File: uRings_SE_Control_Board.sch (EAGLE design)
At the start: 32 parts, among them J1 JACK-THONKICONN, J10 JACK-THONKICONN, J2 JACK-THONKICONN, J3 JACK-THONKICONN, J4 JACK-THONKICONN, J5 JACK-THONKICONN, J6 JACK-THONKICONN, J7 JACK-THONKICONN, J8 JACK-THONKICONN, J9 JACK-THONKICONN, P1 10k, P10 10k, P2 10k, P3 10k, P4 10k, P5 10k, P6 10k, P7 10k, P8 10k, P9 10k

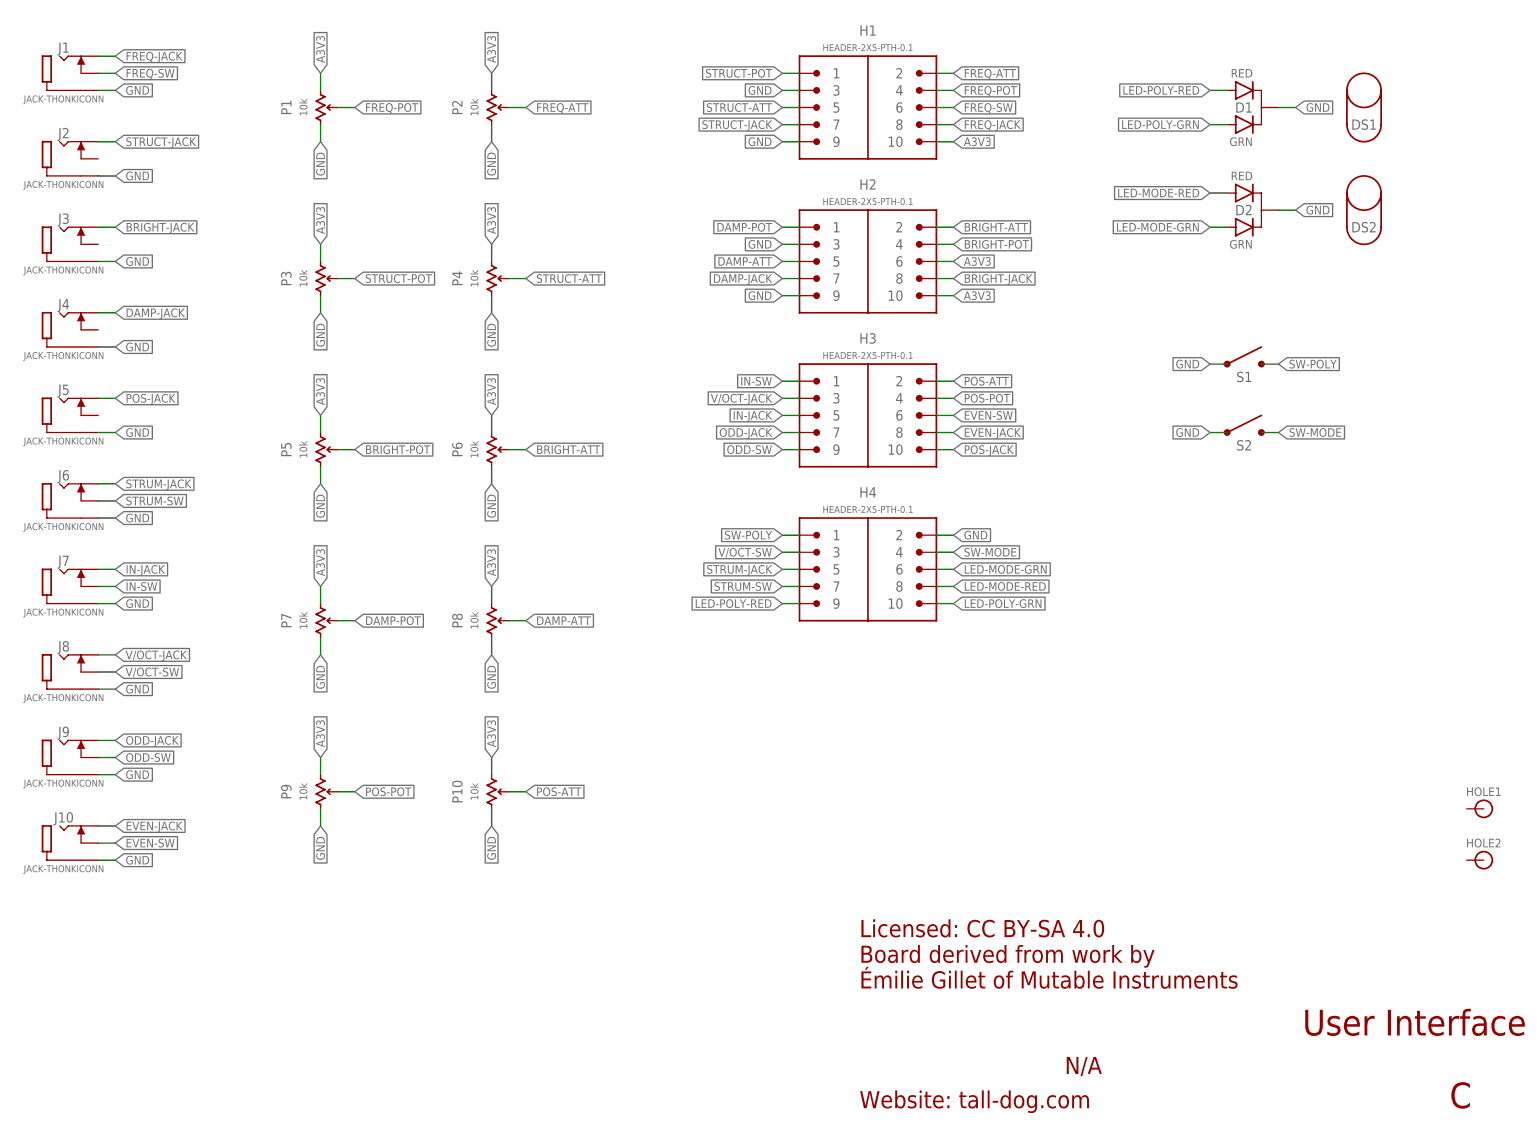
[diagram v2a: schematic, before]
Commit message: updates in preparation for rev D production
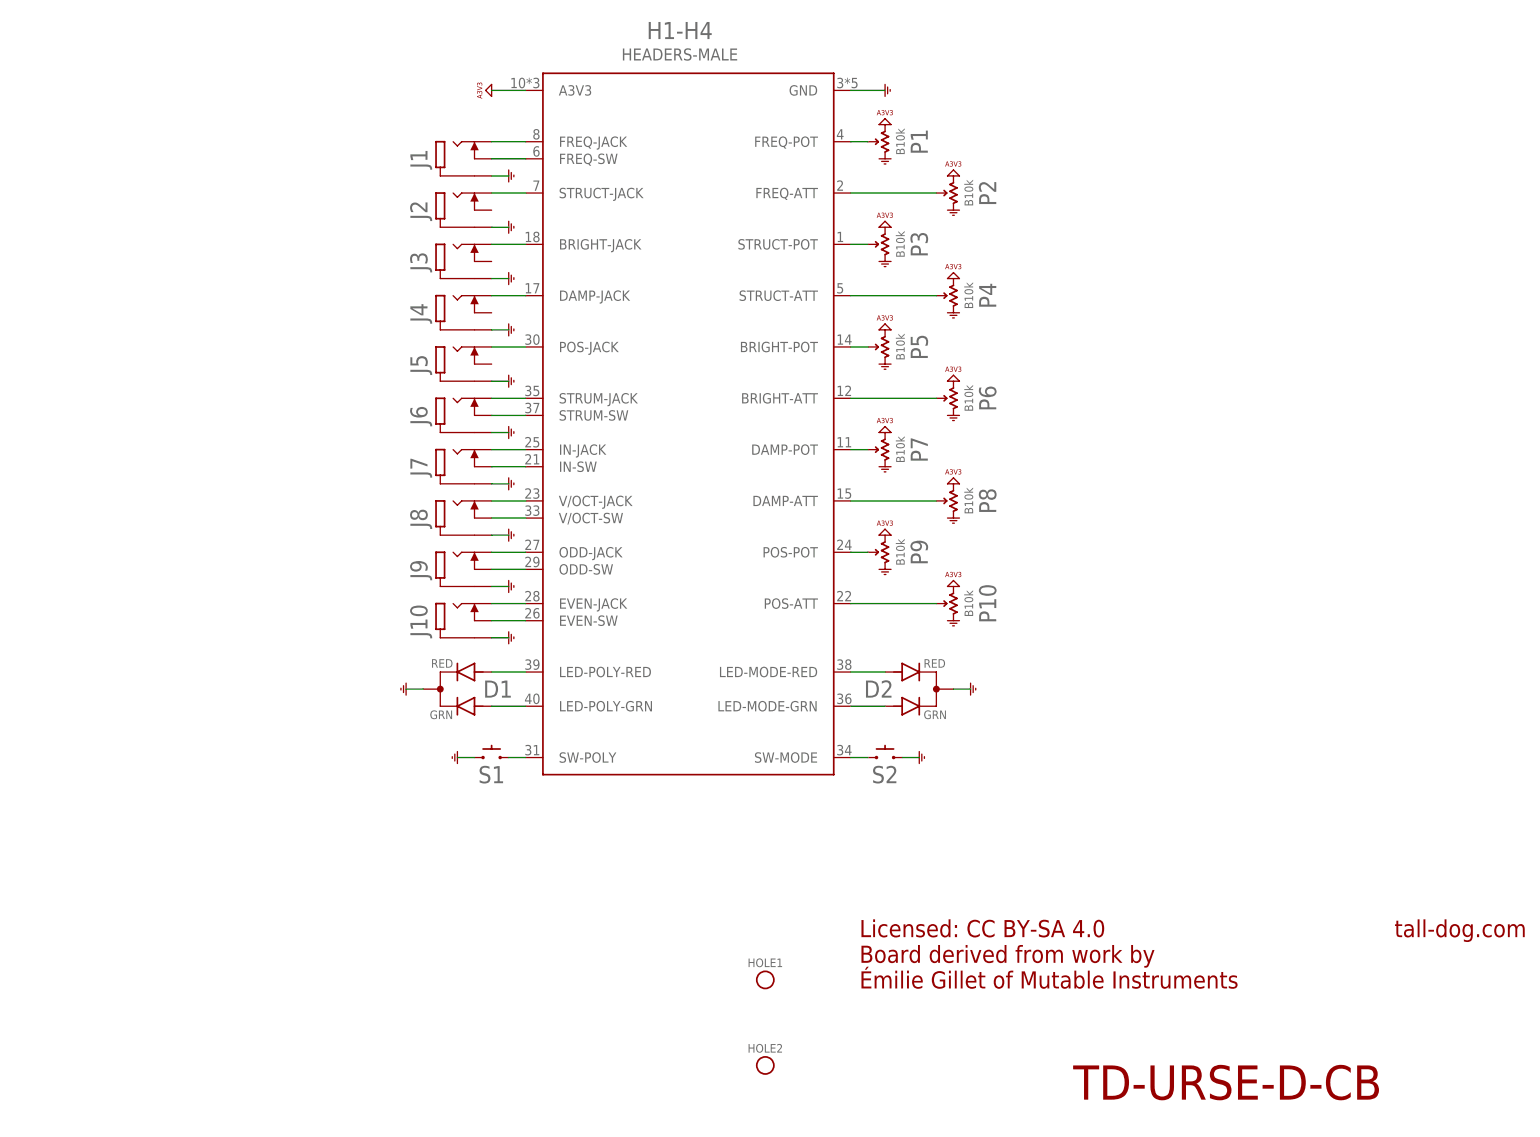
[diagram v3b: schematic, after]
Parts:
- removed DS1, DS2: LED-SPACER, uRings_SE_Library:LED-SPACER
- removed H1, H2, H3, H4: HEADER-2X5-PTH-0.1, uRings_SE_Library:HEADER-2X5-PTH-0.1
- added H1-H4: HEADERS-MALE, uRings_SE_Library:HEADERS-MALE
- D1, D2: value LED-DUAL-PTH -> LED-DUAL; device uRings_SE_Library:LED-DUAL-PTH -> uRings_SE_Library:LED-DUAL
- J1, J10, J2, J3, J4, J5, J6, J7, J8, J9: value JACK-THONKICONN -> JACK; device uRings_SE_Library:JACK-THONKICONN -> uRings_SE_Library:JACK
- P1, P10, P2, P3, P4, P5, P6, P7, P8, P9: value 10k -> B10k; device uRings_SE_Library:POT-ALPS-VERT-PS -> uRings_SE_Library:POT
- S1, S2: value SPST-PTH -> SPST; device uRings_SE_Library:SPST-PTH -> uRings_SE_Library:SPST
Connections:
- net A3V3: now also H1-H4.A3V3; no longer H1.10, H2.10, H2.6
- net BRIGHT-ATT: now also H1-H4.BRIGHT-ATT; no longer H2.2
- net BRIGHT-JACK: now also H1-H4.BRIGHT-JACK; no longer H2.8
- net BRIGHT-POT: now also H1-H4.BRIGHT-POT; no longer H2.4
- net DAMP-ATT: now also H1-H4.DAMP-ATT; no longer H2.5
- net DAMP-JACK: now also H1-H4.DAMP-JACK; no longer H2.7
- net DAMP-POT: now also H1-H4.DAMP-POT; no longer H2.1
- net EVEN-JACK: now also H1-H4.EVEN-JACK; no longer H3.8
- net EVEN-SW: now also H1-H4.EVEN-SW; no longer H3.6
- net FREQ-ATT: now also H1-H4.FREQ-ATT; no longer H1.2
- net FREQ-JACK: now also H1-H4.FREQ-JACK; no longer H1.8
- net FREQ-POT: now also H1-H4.FREQ-POT; no longer H1.4
- net FREQ-SW: now also H1-H4.FREQ-SW; no longer H1.6
- net GND: now also H1-H4.GND; no longer H1.3, H1.9, H2.3, H2.9, H4.2
- net IN-JACK: now also H1-H4.IN-JACK; no longer H3.5
- net IN-SW: now also H1-H4.IN-SW; no longer H3.1
- net LED-MODE-GRN: now also H1-H4.LED-MODE-GRN; no longer H4.6
- net LED-MODE-RED: now also H1-H4.LED-MODE-RED; no longer H4.8
- net LED-POLY-GRN: now also H1-H4.LED-POLY-GRN; no longer H4.10
- net LED-POLY-RED: now also H1-H4.LED-POLY-RED; no longer H4.9
- net ODD-JACK: now also H1-H4.ODD-JACK; no longer H3.7
- net ODD-SW: now also H1-H4.ODD-SW; no longer H3.9
- net POS-ATT: now also H1-H4.POS-ATT; no longer H3.2
- net POS-JACK: now also H1-H4.POS-JACK; no longer H3.10
- net POS-POT: now also H1-H4.POS-POT; no longer H3.4
- net STRUCT-ATT: now also H1-H4.STRUCT-ATT; no longer H1.5
- net STRUCT-JACK: now also H1-H4.STRUCT-JACK; no longer H1.7
- net STRUCT-POT: now also H1-H4.STRUCT-POT; no longer H1.1
- net STRUM-JACK: now also H1-H4.STRUM-JACK; no longer H4.5
- net STRUM-SW: now also H1-H4.STRUM-SW; no longer H4.7
- net SW-MODE: now also H1-H4.SW-MODE; no longer H4.4
- net SW-POLY: now also H1-H4.SW-POLY; no longer H4.1
- net V/OCT-JACK: now also H1-H4.V/OCT-JACK; no longer H3.3
- net V/OCT-SW: now also H1-H4.V/OCT-SW; no longer H4.3
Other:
- note added: "TD-URSE-D-CB"
- note added: "tall-dog.com"
- note removed: "C"
- note removed: "N/A"
- note removed: "User Interface"
- note removed: "Website: tall-dog.com"
- moved on the sheet: J1, J10, J2, J3, J4, J5, J6, J7, J8, J9, P1, P10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
